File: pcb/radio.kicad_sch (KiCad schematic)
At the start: 29 parts, among them J4 AM Antenna, J5 FM Antenna, J6 AudioJack3_SwitchTR, U29 Si4735-D60-GU, U31 TDA1308, Y1 32.768kHz

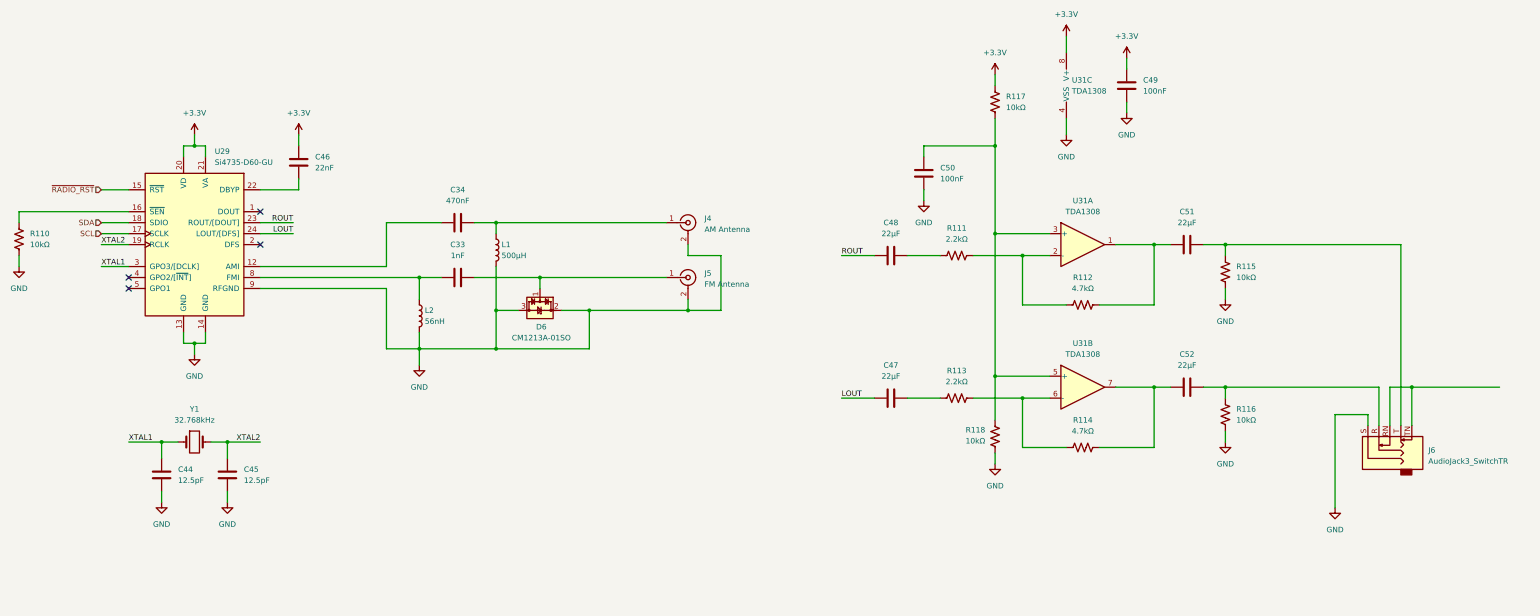
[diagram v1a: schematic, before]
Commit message: w
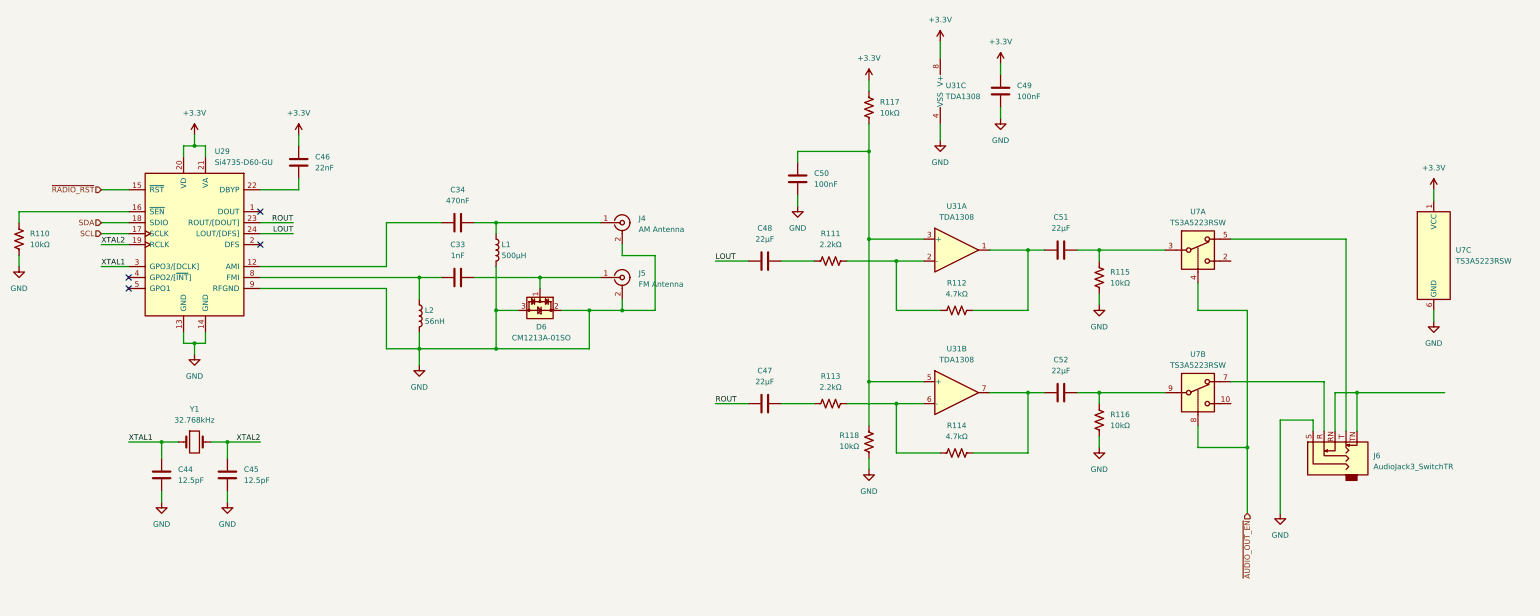
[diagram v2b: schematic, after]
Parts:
- added U7: TS3A5223RSW, Package_DFN_QFN:Texas_RSW0010A_UQFN-10_1.4x1.8mm_P0.4mm, symbol Analog_Switch:TS3A5223RSW
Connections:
- net +3.3V: now also U7.1 (VCC)
- net GND: now also U7.6 (GND)
- net LOUT: now also C48.2; no longer C47.2
- net ROUT: now also C47.2; no longer C48.2
- net at C51.1, R115.1: now also U7.3; no longer J6.T
- net at C52.1, R116.1: now also U7.9; no longer J6.R
- new net: J6.T, U7.5
- new net: J6.R, U7.7
- new net ~{AUDIO_OUT_EN}: U7.4, U7.8
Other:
- moved on the sheet: C47, C48, C49, C50, C51, C52, J4, J5, J6, R111, R112, R113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

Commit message: w
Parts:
- J4, J5: footprint (none) -> Connector_Coaxial:BNC_TEConnectivity_1478204_Vertical
- J6: footprint (none) -> Connector_Audio:Jack_3.5mm_CUI_SJ1-3535NG_Horizontal
- Y1: footprint (none) -> Crystal:Crystal_SMD_3215-2Pin_3.2x1.5mm
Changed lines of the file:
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@@
 			)
 		)
-		(property "Footprint" ""
+		(property "Footprint" "Connector_Audio:Jack_3.5mm_CUI_SJ1-3535NG_Horizontal"
 			(at 345.44 128.27 0)
 			(hide yes)
@@
 			)
 		)
-		(property "Footprint" ""
+		(property "Footprint" "Connector_Coaxial:BNC_TEConnectivity_1478204_Vertical"
 			(at 182.88 74.93 0)
 			(hide yes)
@@
 			)
 		)
-		(property "Footprint" ""
+		(property "Footprint" "Crystal:Crystal_SMD_3215-2Pin_3.2x1.5mm"
 			(at 83.82 125.73 0)
 			(hide yes)
@@
 			)
 		)
-		(property "Footprint" ""
+		(property "Footprint" "Connector_Coaxial:BNC_TEConnectivity_1478204_Vertical"
 			(at 182.88 87.63 0)
 			(hide yes)
